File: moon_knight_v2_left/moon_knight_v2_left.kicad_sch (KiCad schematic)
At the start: 104 parts, among them U1 TRRS, U2 74HCT1G125GW

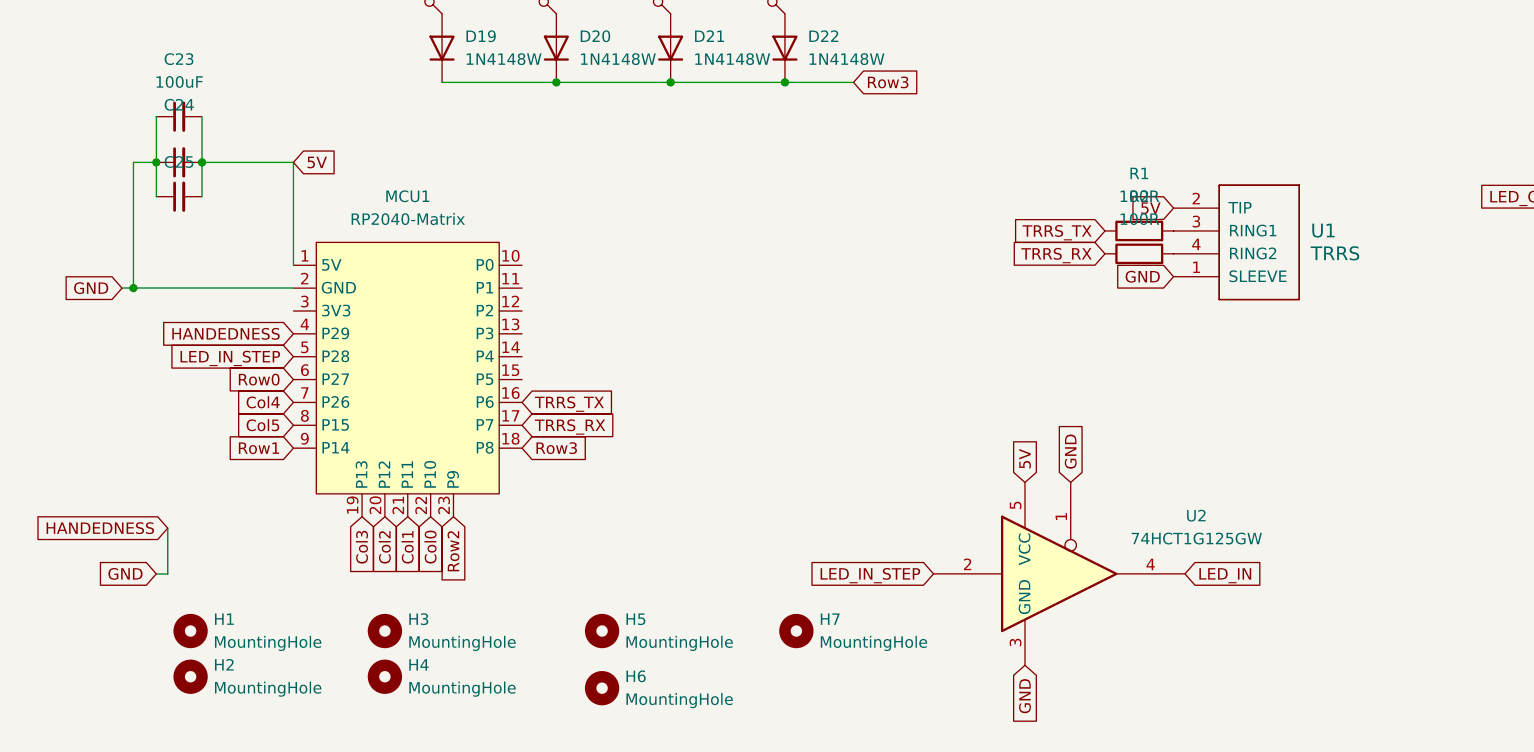
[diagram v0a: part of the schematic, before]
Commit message: Fixes
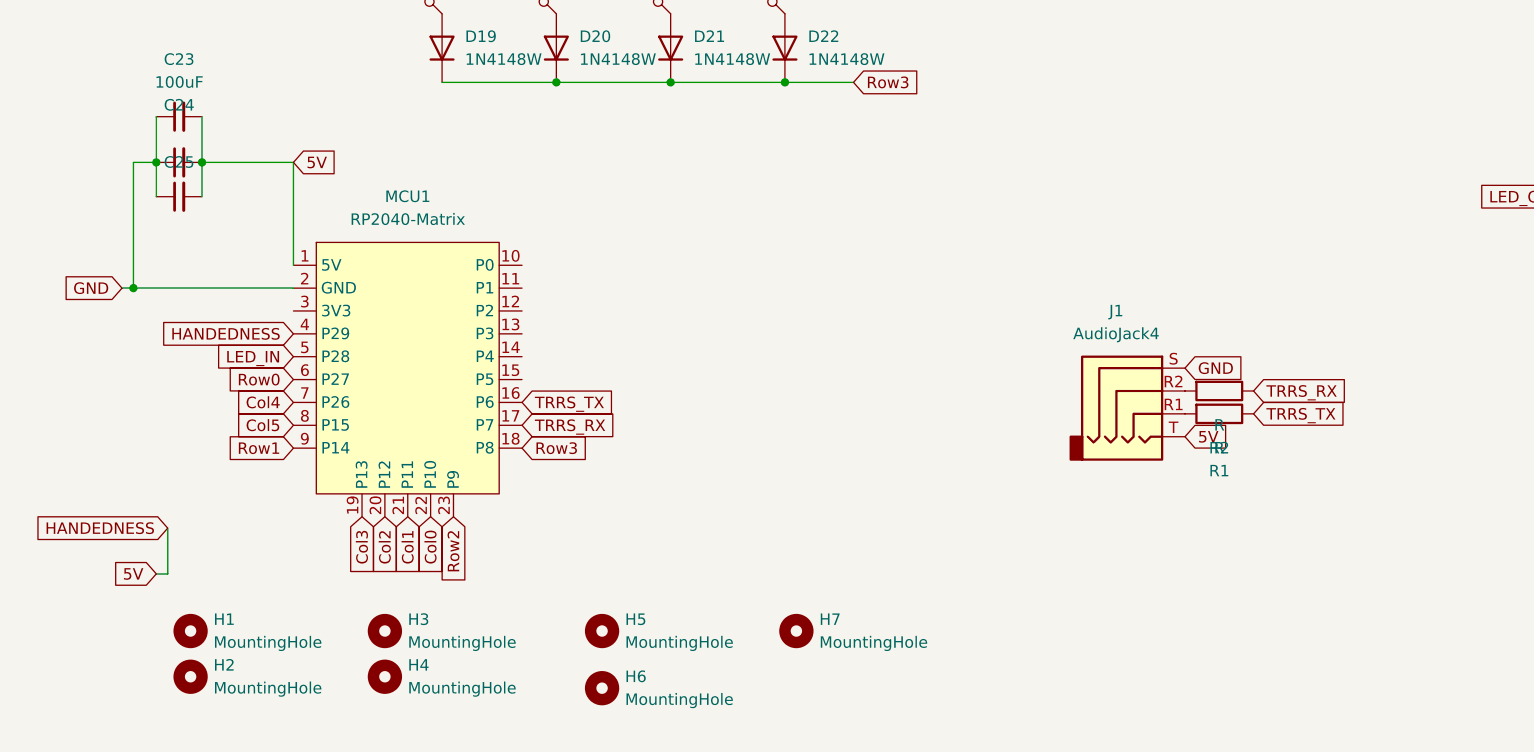
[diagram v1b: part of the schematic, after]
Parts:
- removed R1, R2: 100R, Resistor_SMD:R_1206_3216Metric_Pad1.30x1.75mm_HandSolder, symbol ScottoKeebs:Placeholder_Resistor
- removed U1: TRRS, ScottoKeebs_Components:TRRS_PJ-320A, symbol ScottoKeebs:Placeholder_TRRS
- removed U2: 74HCT1G125GW, Package_TO_SOT_SMD:SOT-23-5, symbol 74xGxx:SN74LVC1G125DBV
- added J1: AudioJack4, PCM_marbastlib-xp-various:CON_MJ-4PP-9_Reversible, symbol Connector_Audio:AudioJack4
- added R1, R2: R, Resistor_SMD:R_1206_3216Metric_Pad1.30x1.75mm_HandSolder, symbol Device:R
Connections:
- net LED_IN_STEP is gone; now on net LED_IN: MCU1.5 (P28)
- net 5V: now also MCU1.4 (P29), J1.T
- net GND: now also J1.S; no longer MCU1.4 (P29)
- net TRRS_RX: now also R2.1
- net TRRS_TX: now also R1.1
- new net: J1.R2, R2.2
- new net: J1.R1, R1.2
